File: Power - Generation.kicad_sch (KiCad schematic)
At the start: 1 part, among them U3 TPSM63603RDHR

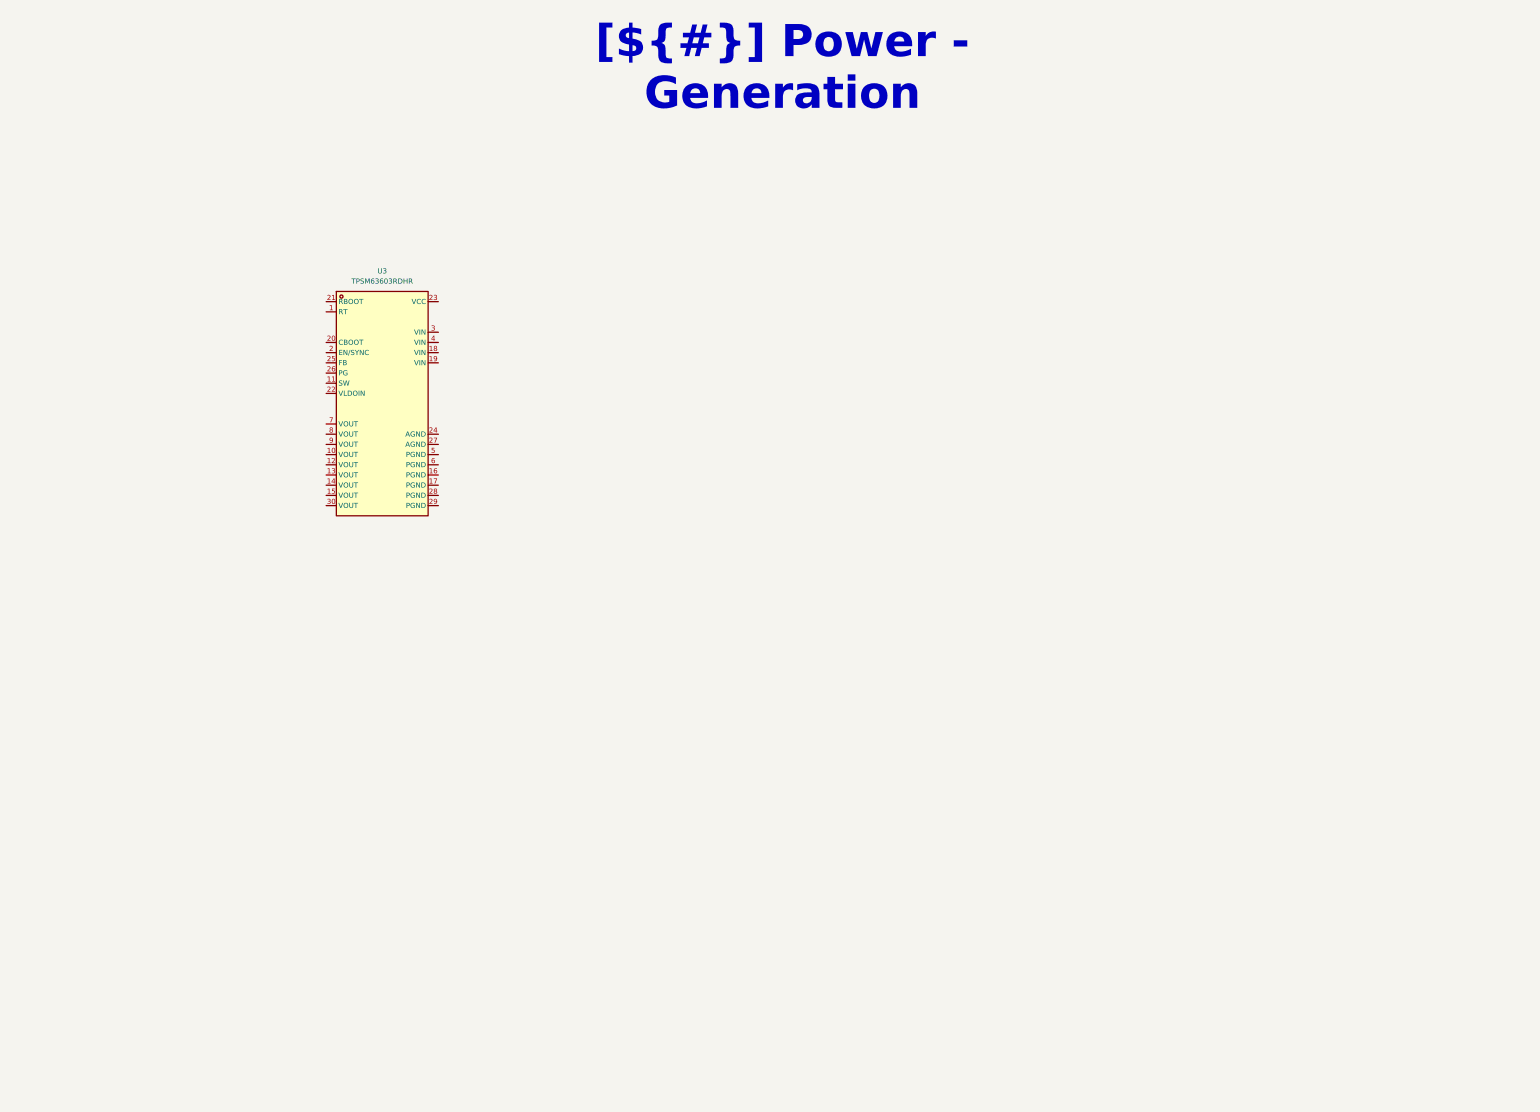
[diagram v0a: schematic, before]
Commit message: [07/07/2026][Power - Generation] Update
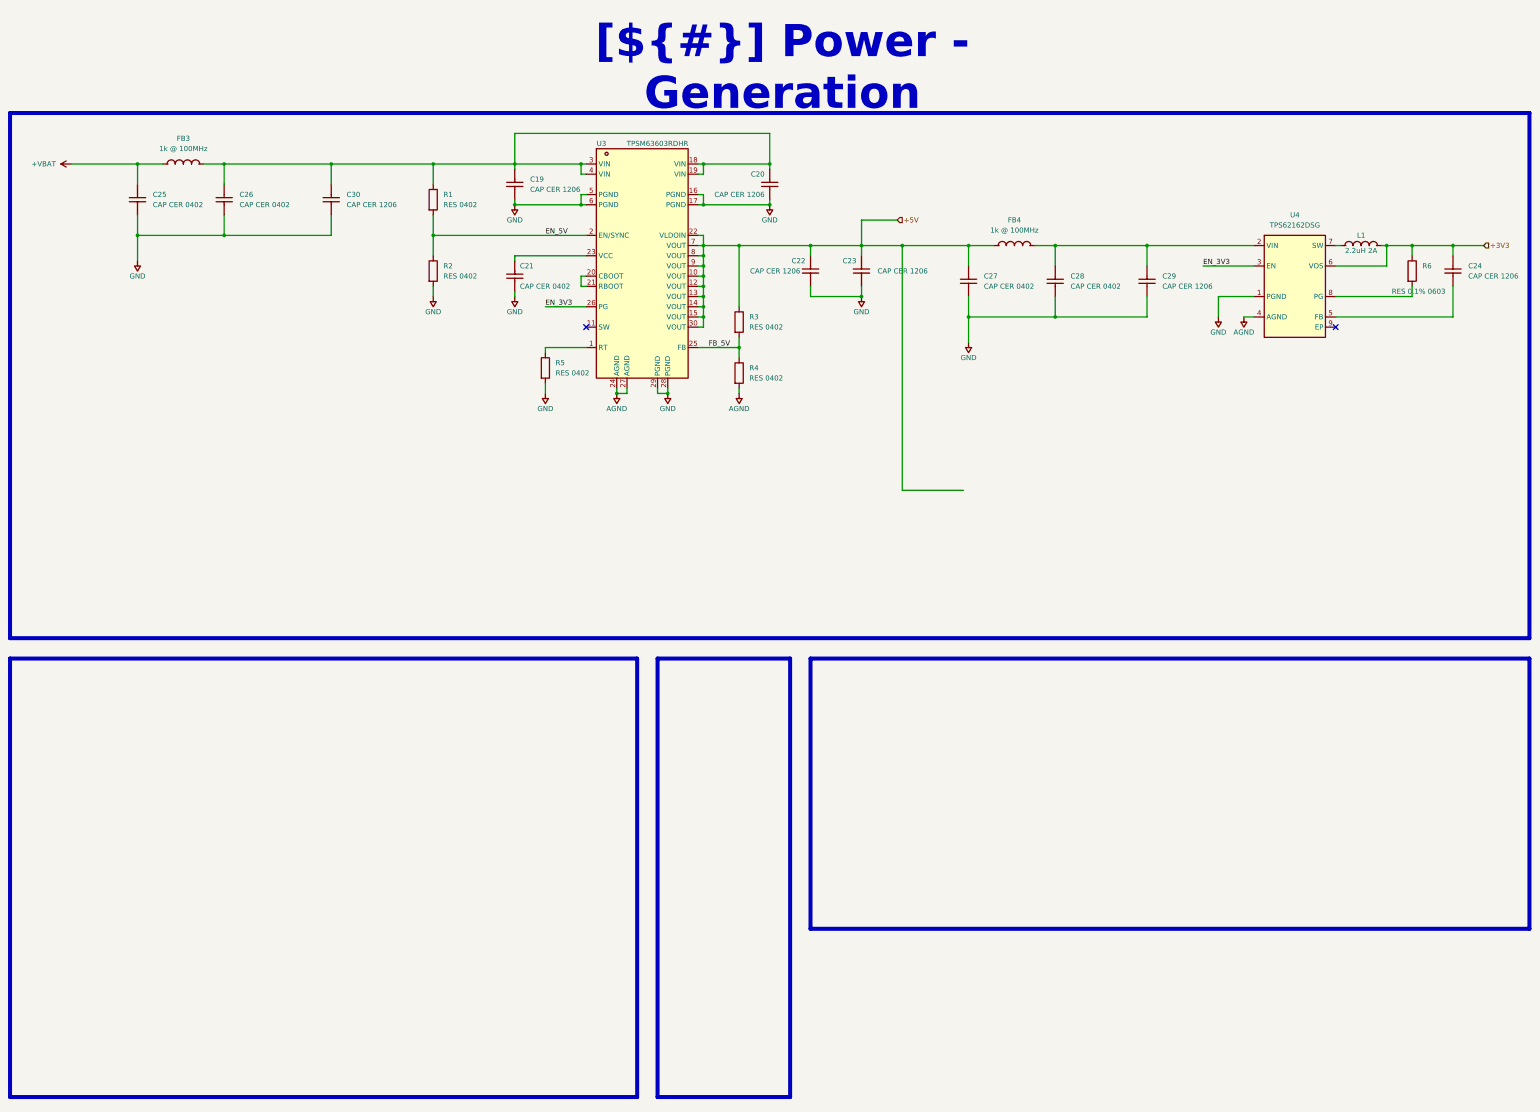
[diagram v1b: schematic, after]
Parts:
- removed U3: TPSM63603RDHR, Duc_Library:QFN-30_L6.0-W4.0-P0.50_TLVM13630RDHR, symbol Duc_Library:TPSM63603RDHR
- added C19, C20, C22, C23, C24, C29, C30: CAP CER 1206, Duc_Library:C1206, symbol Duc-Capacitors:CAP CER 1206
- added C21, C25, C26, C27, C28: CAP CER 0402, Duc_Library:C0402, symbol Duc-Capacitors:CAP CER 0402
- added FB3, FB4: 1k @ 100MHz, Duc_Library:L0805, symbol Duc-Inductors:PBBHAQ2012H-102T10
- added L1: ANR3015T2R2M, Duc:IND-SMD_L3.0-W3.0_SMNR3015, symbol Duc-Inductors:ANR3015T2R2M
- added R1, R2, R3, R4, R5: RES 0402, Duc_Library:R0402, symbol Duc-Resistors:RES SMD 0402
- added R6: RES 0.1% 0603, Duc:R0603, symbol Duc-Resistors:RES SMD 0603
- added U3: TPSM63603RDHR, Duc_Library:QFN-30_L6.0-W4.0-P0.50_TLVM13630RDHR, symbol Duc-Power:TPSM63603RDHR
- added U4: TPS62162DSG, Duc:WSON-8_L2.0-W2.0-P0.50-TL-EP, symbol Duc-Power:TPS62162DSG
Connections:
- new net: L1.1, U4.7 (SW)
- new net: R5.2, U3.1 (RT)
- new net: C19.2, C20.2, C26.2, C30.2, FB3., R1.2, U3.18 (VIN), U3.19 (VIN), U3.3 (VIN), U3.4 (VIN)
- new net: C21.2, U3.23 (VCC)
- new net: C28.2, C29.2, FB4., U4.2 (VIN)
- new net: C24.1, U4.5 (FB)
- new net: R6.1, U4.8 (PG)
- new net: U3.20 (CBOOT), U3.21 (RBOOT)
- new net +3V3: C24.2, L1.2, R6.2, U4.6 (VOS)
- new net +5V: C22.2, C23.2, C27.2, FB4., R3.2, U3.10 (VOUT), U3.12 (VOUT), U3.13 (VOUT), U3.14 (VOUT), U3.15 (VOUT), U3.22 (VLDOIN), U3.30 (VOUT), U3.7 (VOUT), U3.8 (VOUT), U3.9 (VOUT)
- new net +VBAT: C25.2, FB3.
- new net AGND: R4.1, U3.24 (AGND), U3.27 (AGND), U4.4 (AGND)
- new net EN_3V3: U3.26 (PG), U4.3 (EN)
- new net EN_5V: R1.1, R2.2, U3.2 (EN/SYNC)
- new net FB_5V: R3.1, R4.2, U3.25 (FB)
- new net GND: C19.1, C20.1, C21.1, C22.1, C23.1, C25.1, C26.1, C27.1, C28.1, C29.1, C30.1, R2.1, R5.1, U3.16 (PGND), U3.17 (PGND), U3.28 (PGND), U3.29 (PGND), U3.5 (PGND), U3.6 (PGND), U4.1 (PGND)
- no-connect marks 0 -> 2

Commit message: Update Power Generation Schematic
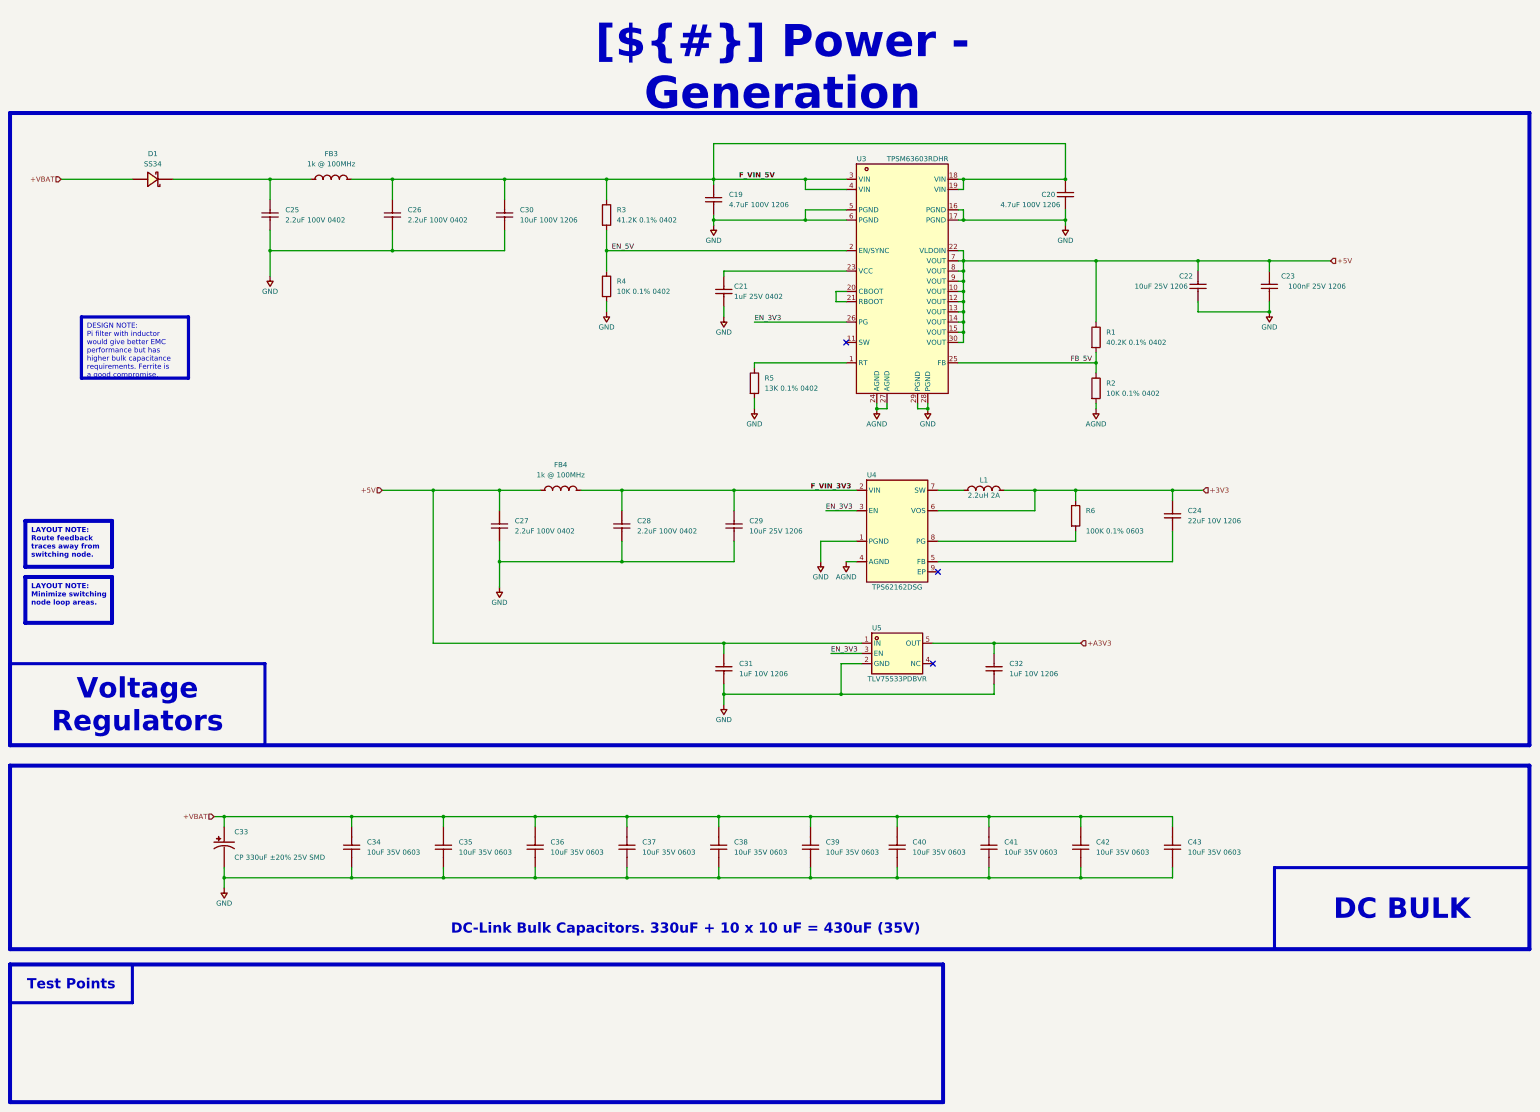
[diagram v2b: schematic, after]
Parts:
- added C31, C32: 1uF 10V 1206, Duc_Library:C1206, symbol Duc-Capacitors:CAP CER 1206
- added C33: 25SVPF330M, Duc:CAP-SMD_BD10.0-L10.3-W10.3-LS11.0-FD, symbol Duc-Capacitors:25SVPF330M
- added C34, C35, C36, C37, C38, C39, C40, C41, C42, C43: 10uF 35V 0603, Duc:C0603, symbol Duc-Capacitors:CAP CER 0603
- added D1: SS34, Duc:SMA_L4.3-W2.5-LS5.0-RD, symbol Duc-Diodes:SS34
- added U5: TLV75533PDBVR, Duc:SOT-23-5_L3.0-W1.7-P0.95-LS2.8-BR, symbol Duc-Power:TLV75533PDBVR
- C19, C20: value CAP CER 1206 -> 4.7uF 100V 1206
- C21: value CAP CER 0402 -> 1uF 25V 0402
- C22, C29: value CAP CER 1206 -> 10uF 25V 1206
- C23: value CAP CER 1206 -> 100nF 25V 1206
- C24: value CAP CER 1206 -> 22uF 10V 1206
- C25, C26, C27, C28: value CAP CER 0402 -> 2.2uF 100V 0402
- C30: value CAP CER 1206 -> 10uF 100V 1206
- R1: value RES 0402 -> 40.2K 0.1% 0402
- R2, R4: value RES 0402 -> 10K 0.1% 0402
- R3: value RES 0402 -> 41.2K 0.1% 0402
- R5: value RES 0402 -> 13K 0.1% 0402
- R6: value RES 0.1% 0603 -> 100K 0.1% 0603
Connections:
- net +5V: now also R1.2, C31.2, U5.1 (IN); no longer R3.2
- net +VBAT: now also C33.1, C34.1, C35.1, C36.1, C37.1, C38.1, C39.1, C40.1, C41.1, C42.1, C43.1, D1.2 (A); no longer C25.2, FB3.
- net AGND: now also R2.1; no longer R4.1
- net EN_3V3: now also U5.3 (EN)
- net EN_5V: now also R3.1, R4.2; no longer R1.1, R2.2
- net FB_5V: now also R1.1, R2.2; no longer R3.1, R4.2
- net GND: now also R4.1, C31.1, C32.1, C33.2, C34.2, C35.2, C36.2, C37.2, C38.2, C39.2, C40.2, C41.2, C42.2, C43.2, U5.2 (GND); no longer R2.1
- net F_VIN_5V: now reaches C19.2, C20.2, C26.2, C30.2, FB3., U3.18 (VIN), U3.19 (VIN), U3.3 (VIN), U3.4 (VIN)
- net F_VIN_5V: now also R3.2; no longer R1.2
- net F_VIN_3V3: now reaches C28.2, C29.2, FB4., U4.2 (VIN)
- new net: C25.2, D1.1 (C), FB3.
- new net +A3V3: C32.2, U5.5 (OUT)
- no-connect marks 2 -> 3
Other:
- moved on the sheet: C19, C20, C21, C22, C23, C24, C25, C26, C27, C28, C29, C30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
